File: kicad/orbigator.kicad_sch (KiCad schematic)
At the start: 40 parts, among them J1 Conn_01x01, J10 Conn_01x01, J11 Conn_01x01, J12 Conn_01x01, J13 Conn_01x01, J14 Conn_01x01, J15 Conn_01x01, J16 Conn_01x01, J17 Conn_01x01, J18 Conn_01x01, J19 Conn_01x01, J2 Conn_01x01, J20 Conn_01x01, J21 Conn_01x01, J22 Conn_01x01, J23 Conn_01x01, J24 Conn_01x01, J25 Conn_01x01, J26 Conn_01x01, J27 Barrel_Jack_Switch, J28 Conn_01x01, J29 Conn_01x01, J3 Conn_01x01, J30 Conn_01x01, J4 Conn_01x01, J5 Conn_01x01, J6 Conn_01x01, J7 Conn_01x01, J8 Conn_01x01, J9 Conn_01x01, M1 DYNAMIXEL_1, M2 DYNAMIXEL_2, U1 Pico_2, U2 74LS126, U3 DC_polarity

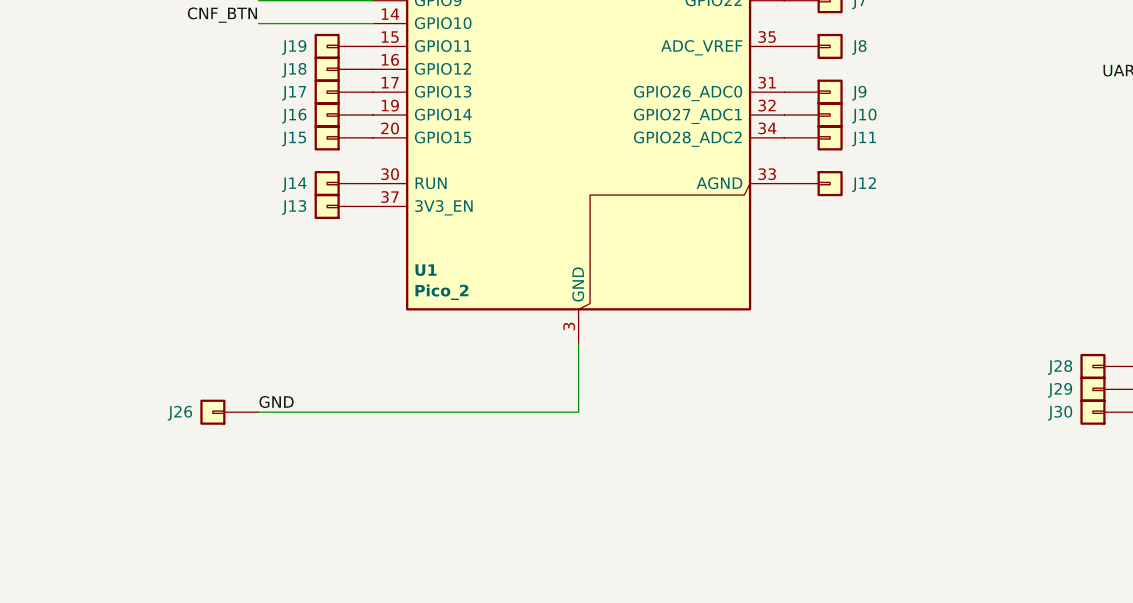
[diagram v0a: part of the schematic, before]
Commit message: PCB layout done
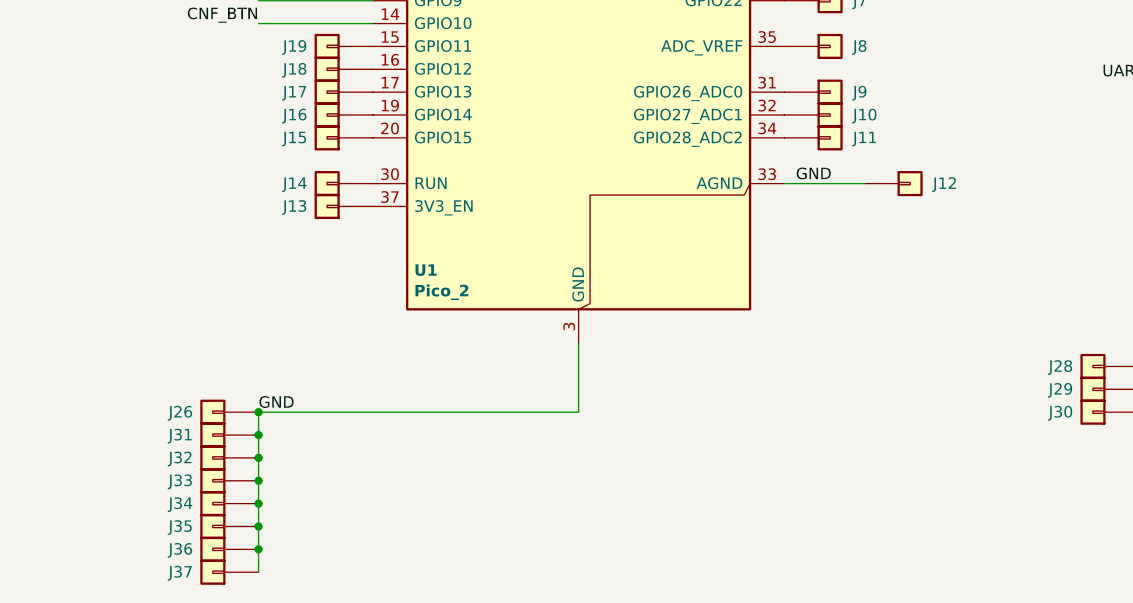
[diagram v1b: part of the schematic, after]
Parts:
- added J31, J32, J33, J34, J35, J36, J37: Conn_01x01, orbigator:PinHeader_1x01_P2.54mm_Vertical, symbol orbigator:Conn_01x01_1
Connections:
- net GND: now also J12.1 (Pin_1), U1.33 (AGND), J31.1 (Pin_1), J32.1 (Pin_1), J33.1 (Pin_1), J34.1 (Pin_1), J35.1 (Pin_1), J36.1 (Pin_1), J37.1 (Pin_1)
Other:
- moved on the sheet: J12
